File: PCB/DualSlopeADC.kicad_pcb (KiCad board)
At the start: 2 copper layers, 45 x 72 mm, 25 parts, among them J1 Conn_01x02_Pin, J2 Conn_01x02_Pin, J3 Conn_01x02_Pin, J4 Conn_01x02_Pin, J5 Conn_01x02_Pin, J6 Conn_01x02_Pin, J7 Conn_01x02_Pin, J8 Conn_01x02_Pin, U1 CH32V003FxPx, U2 ADR4533, U3 AD8605ARTZ-R2, U4 ADG419BRM, U5 LTC6752xSC6-4, U6 CA56-12EWA

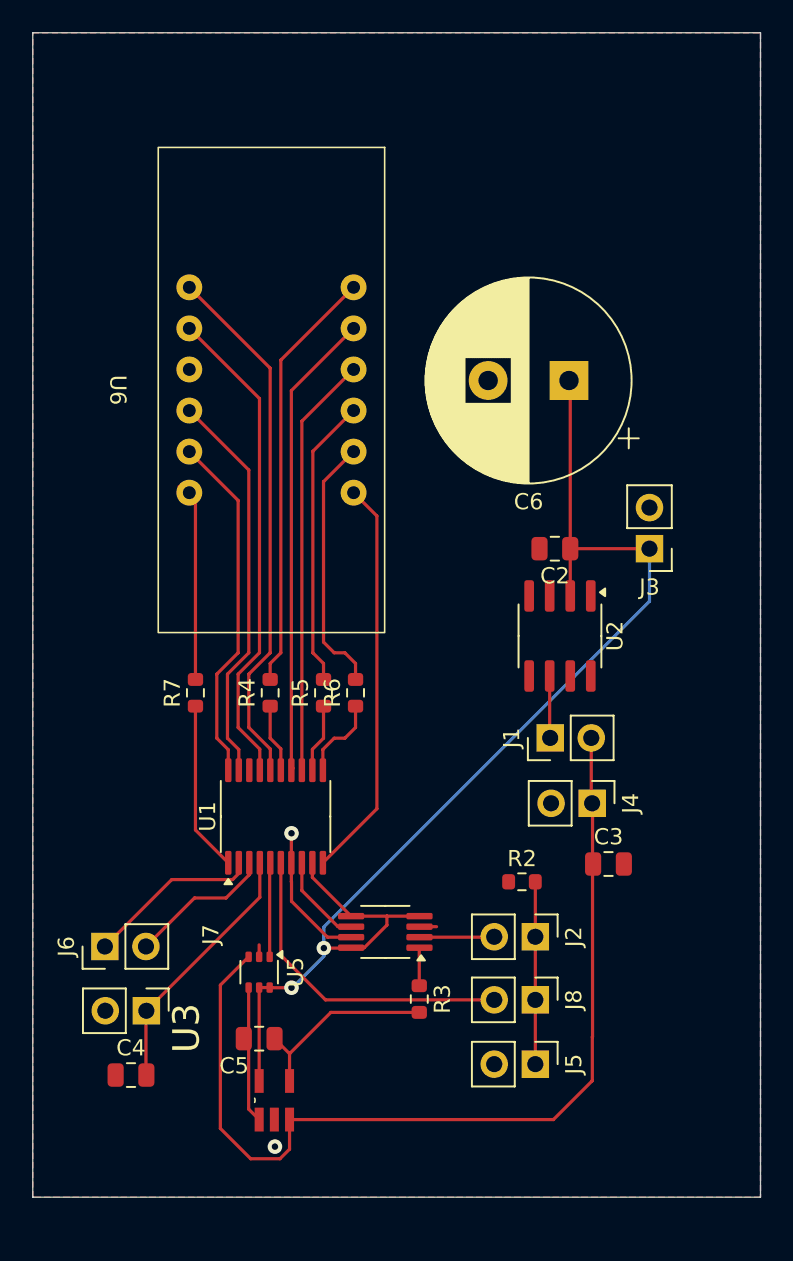
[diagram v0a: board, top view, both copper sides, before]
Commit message: platine fertig
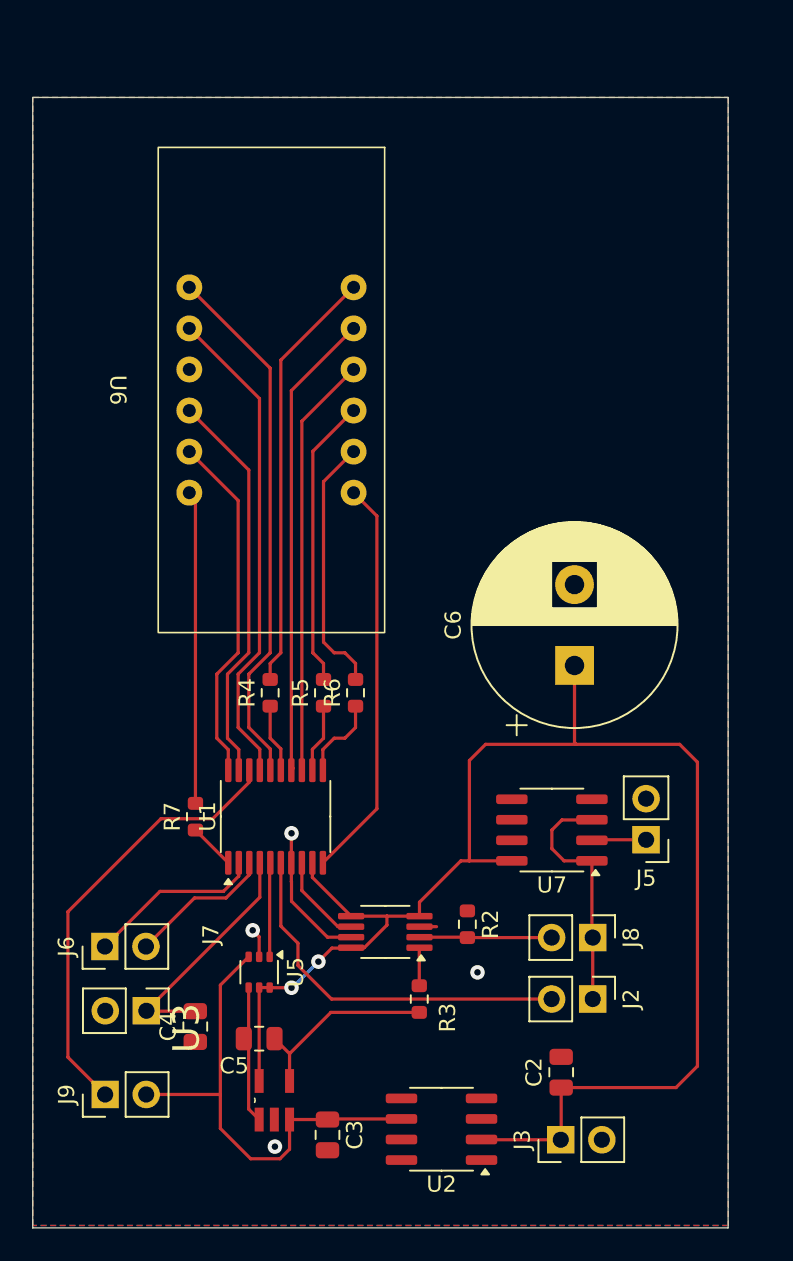
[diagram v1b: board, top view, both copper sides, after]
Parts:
- removed J1, J4: Conn_01x02_Pin, Connector_PinHeader_2.54mm:PinHeader_1x02_P2.54mm_Vertical
- added J9: Conn_01x02_Pin, Connector_PinHeader_2.54mm:PinHeader_1x02_P2.54mm_Vertical, F.Cu at (186.5, 125.7)
- added U7: AD8656, Package_SO:SOIC-8_3.9x4.9mm_P1.27mm, F.Cu at (214.1, 109.3)
- moved J3 37.0 mm to (214.7, 128.4), turned to 90 degrees
- moved C2 32.4 mm to (214.7, 124.3), turned to 90 degrees
- moved U2 31.4 mm to (207.3, 127.8), turned to 180 degrees
- moved C3 24.1 mm to (200.2, 128.2), turned to -90 degrees
- moved C6 17.6 mm to (215.5, 99.1), turned to 90 degrees
- moved J5 15.5 mm to (219.9, 109.9), turned to 180 degrees
- moved R7 7.66 mm to (192.1, 108.5)
- moved J2 5.24 mm to (216.6, 119.8)
- moved J8 5.24 mm to (216.6, 116.0)
- moved C4 4.98 mm to (192.1, 121.5), turned to 90 degrees
- moved R2 4.28 mm to (208.9, 115.1), turned to -90 degrees
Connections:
- J2 pad 1: Vin -> Net-(J2-Pin_1)
- J2 pad 2: Net-(J2-Pin_2) -> ADC_IN_MC
- J8 pad 1: Vin -> Net-(J2-Pin_1)
- J8 pad 2: Net-(J8-Pin_2) -> ADC_IN_EXT
- R2 pad 2: Vin -> ADC_IN_EXT
- U1 pad 6: Net-(J8-Pin_2) -> ADC_IN_MC
- U2 pad 6: Net-(J1-Pin_1) -> VCC_3V3
- U4 pad 2: Net-(J2-Pin_2) -> ADC_IN_EXT
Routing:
- net VCC_3V3: track 59.5 -> 30.0 mm
- net SWIO: track 0.00 -> 27.5 mm
- net ADC_IN_MC: track 0.00 -> 23.3 mm
- net Net-(J8-Pin_2): track 20.1 -> 0.00 mm
- net VCC_5V: track 76.2 -> 94.3 mm
- net Net-(J2-Pin_1): track 0.00 -> 15.2 mm
- net ADC_IN_EXT: track 0.00 -> 8.18 mm
- net Vin: track 11.3 -> 3.41 mm
- net Net-(U1-PD4): track 10.5 -> 2.87 mm
- net DIG_6: track 11.7 -> 19.4 mm
- net Net-(J2-Pin_2): track 4.63 -> 0.00 mm
- net Net-(J1-Pin_1): track 3.91 -> 0.00 mm
- net GND: track 10.7 -> 11.7 mm, vias 2 -> 4
- net NRST: track 16.1 -> 15.1 mm
- net Tx: track 10.8 -> 11.6 mm
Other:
- board size 45 x 72 mm -> 43 x 69.9 mm
